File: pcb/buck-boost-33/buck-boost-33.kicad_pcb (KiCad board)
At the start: 2 copper layers, 23.5 x 17.5 mm, 14 parts, among them IC1 TP4056, J1 BATT, J2 buck-boost-conn, J3 PWR, U1 TPS63031DSKT

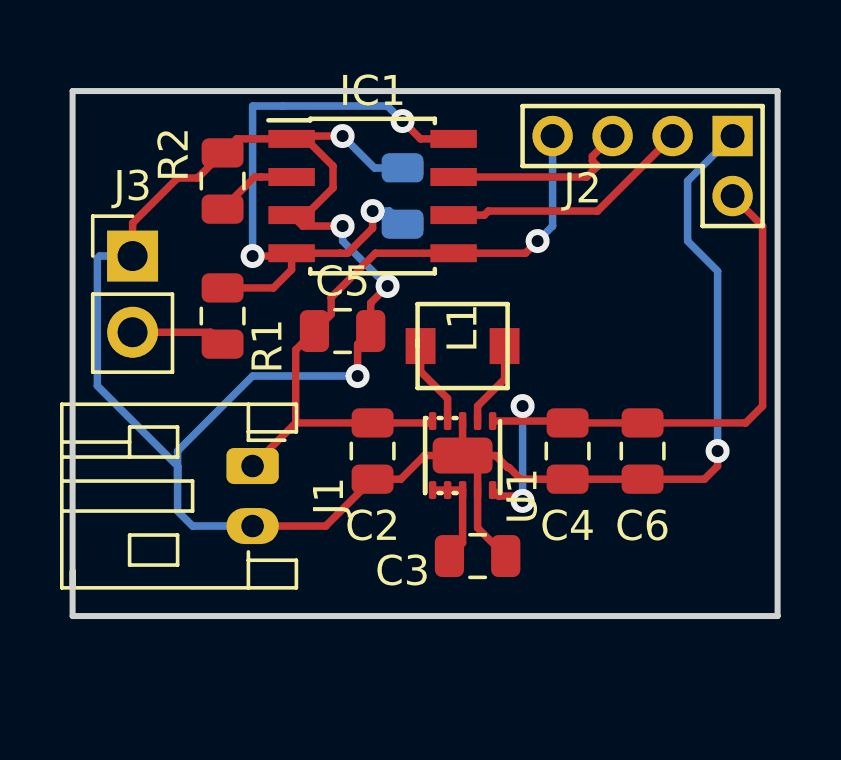
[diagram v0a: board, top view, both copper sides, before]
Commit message: rework with new footprints
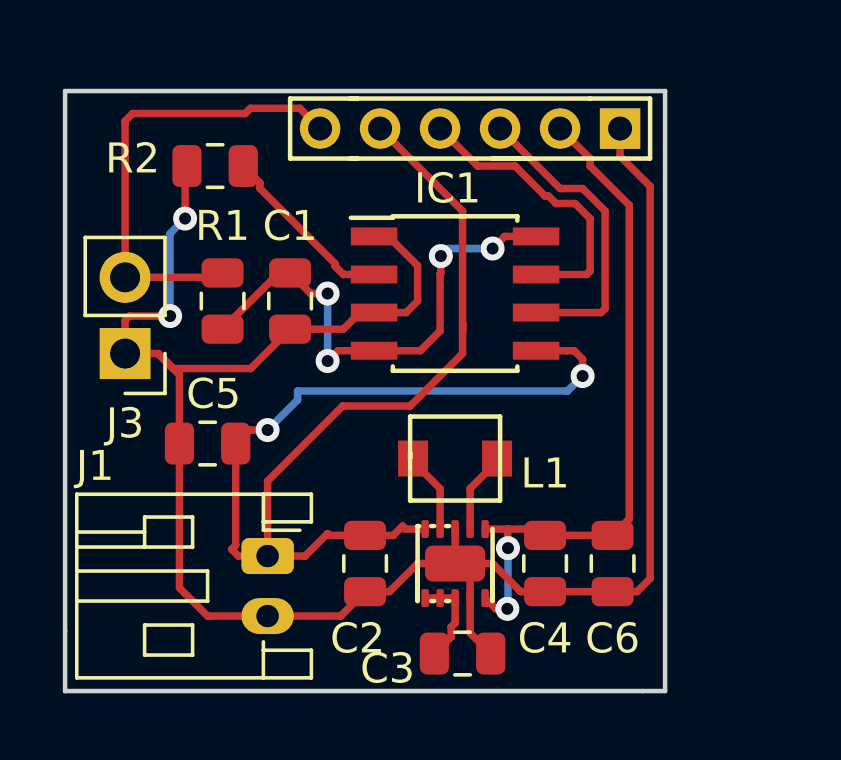
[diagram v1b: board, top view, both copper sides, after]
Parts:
- C1: moved to F.Cu
- L1: footprint coil:Murata 1266AS-H-1R5N=P2 -> coil:Murata_1266AS-H-1R5N=P2
- moved C5 5.86 mm to (94.0, 85.2), turned to 180 degrees
- moved J2 5.76 mm to (102.8, 79.8)
- moved C1 5.13 mm to (96.8, 80.5), turned to 270 degrees
- moved IC1 4.26 mm to (102.2, 80.2)
- moved C6 3.88 mm to (107.5, 89.2)
- moved C4 3.82 mm to (105.2, 89.2)
- moved C2 3.76 mm to (99.2, 89.2)
- moved L1 3.76 mm to (102.2, 85.8)
- moved C3 3.29 mm to (102.5, 92.2)
- moved J3 3.26 mm to (91.2, 82.2), turned to 180 degrees
- moved U1 3.26 mm to (102.2, 89.2)
- moved J1 3.04 mm to (96.0, 89.0)
- moved R2 0.56 mm to (94.2, 76.0), turned to 180 degrees
- moved R1 0.50 mm to (94.5, 80.5), turned to 270 degrees
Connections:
- net Net-(C4-Pad2) renamed /3.3V
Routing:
- net BATT: track 22.7 -> 45.3 mm, vias 1 -> 2
- net +5V: track 3.16 -> 15.5 mm
- net GND: track 79.5 -> 67.4 mm, vias 5 -> 2
- net Net-(C1-Pad1): track 21.4 -> 16.9 mm, vias 3 -> 4
- net CHRG: track 6.30 -> 9.84 mm
- net Net-(IC1-Pad2): track 2.74 -> 6.02 mm
- net STDBY: track 8.39 -> 10.2 mm
- net /3.3V: track 21.5 -> 22.7 mm
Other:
- board size 23.5 x 17.5 mm -> 20 x 20 mm
